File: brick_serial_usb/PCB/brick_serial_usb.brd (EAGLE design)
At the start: 27.9 x 39.4 mm, 15 parts, among them U1 FT232RL-SSOP28

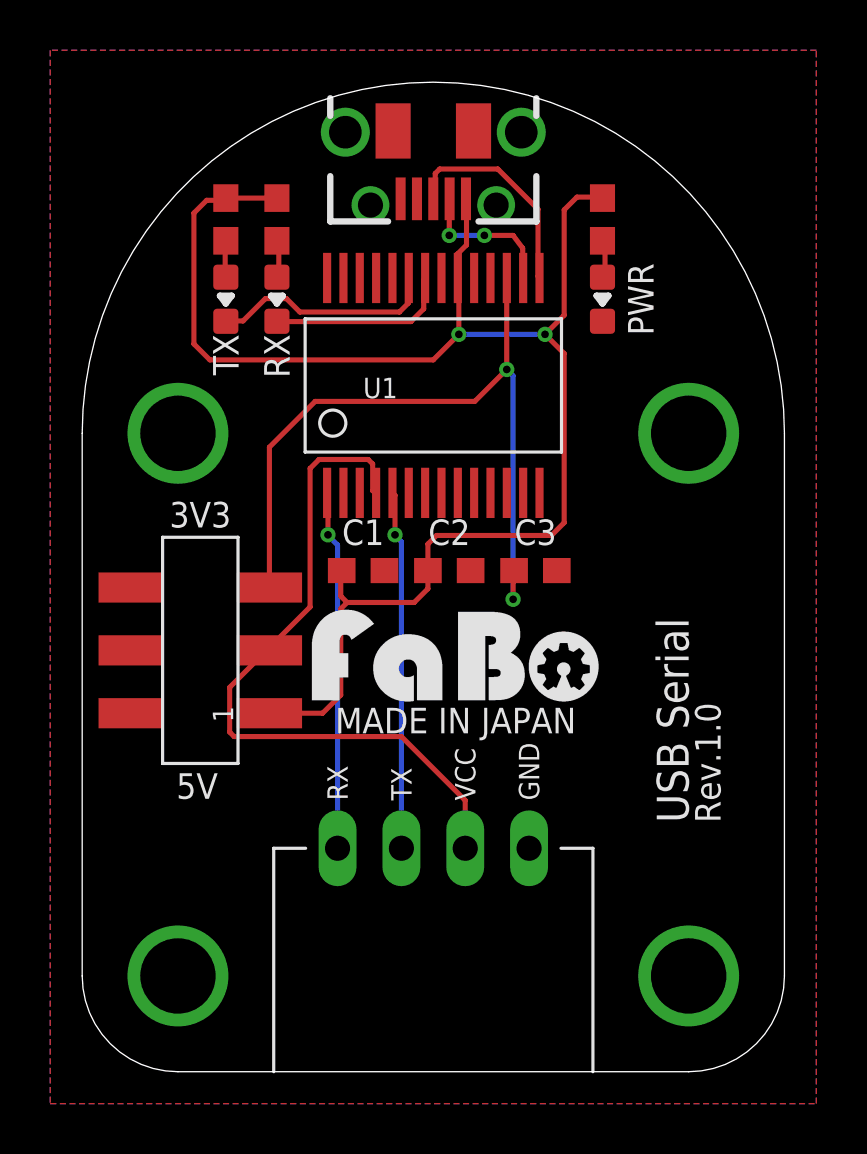
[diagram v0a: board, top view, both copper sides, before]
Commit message: refine board brick_serial_usb
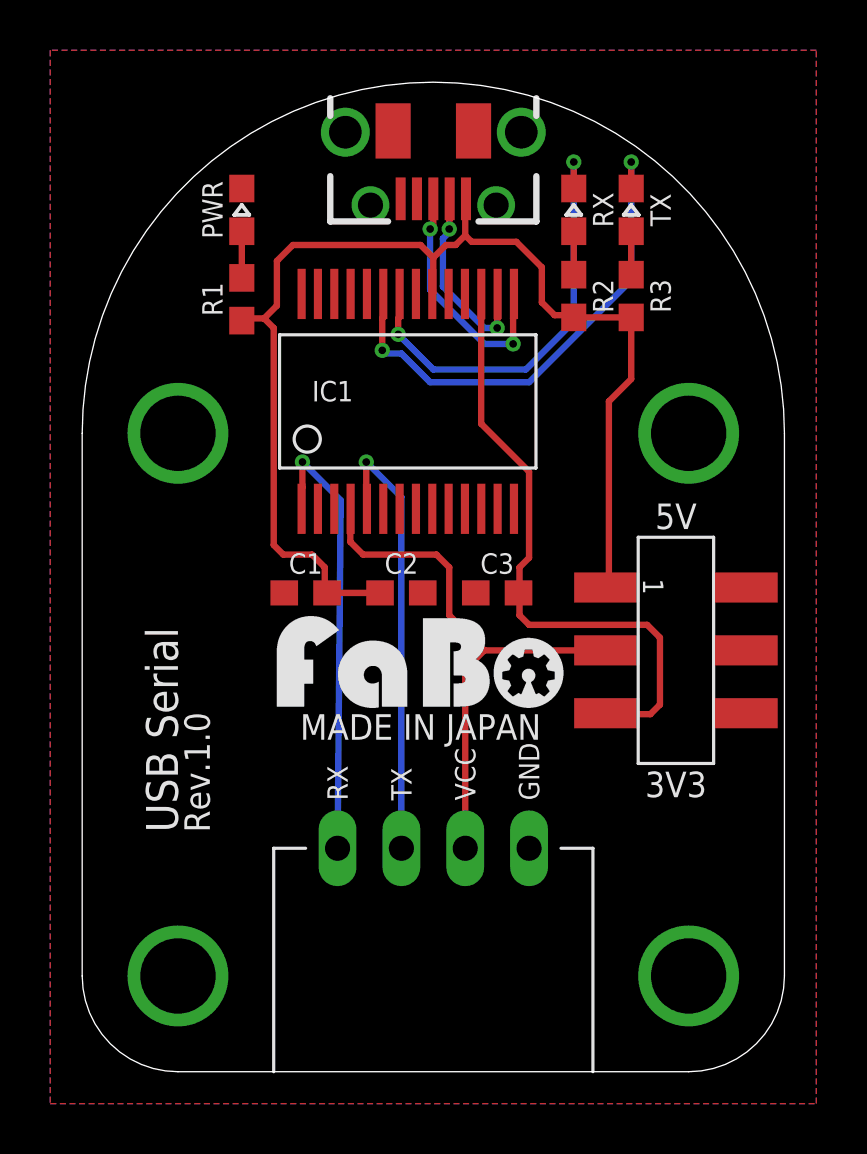
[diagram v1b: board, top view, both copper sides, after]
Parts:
- removed U1: FT232RL-SSOP28, gclue:SSOP28
- added IC1: FT232RL-SSOP28, FaBo-etc:SSOP28
- C1, C2, C3: device gclue:EIA0603 -> FaBo-etc:EIA0603
- J1: device FaBo-etc:BRICK_SERIAL -> FaBo-Template:FABO_BRICK_SERIAL
- JP1: device gclue:USB_B_MICRO -> FaBo-etc:USB_B_MICRO
- PWR, RX, TX: device gclue:EIA0603-LED -> FaBo-etc:EIA0603-LED
- R1, R2, R3: value (none) -> 220; device gclue:EIA0603 -> FaBo-etc:EIA0603
- SW1: device gclue:C&K_JS202011SCQN -> FaBo-etc:C&K_JS202011SCQN
- U$5: device FaBo:LOGO_FABO_M -> FaBo-etc:LOGO_OSHW_T_M_BOTTOM
- U$6: device gclue:LOGO_OSHW_T_M_BOTTOM -> FaBo-etc:LOGO_FABO_M
- moved SW1 18.9 mm to (23.6, 16.8), turned to 0 degrees
- moved TX 16.5 mm to (21.8, 34.3), turned to 90 degrees
- moved PWR 14.8 mm to (6.35, 34.3), turned to 90 degrees
- moved R1 14.7 mm to (6.35, 30.7), turned to 270 degrees
- moved R3 14.4 mm to (21.8, 30.9), turned to 270 degrees
- moved R2 14.2 mm to (19.6, 30.9), turned to 270 degrees
- moved RX 12.3 mm to (19.6, 34.3), turned to 90 degrees
- moved U$5 9.95 mm to (14.0, 4.83)
- moved U$6 9.16 mm to (13.5, 14.5)
- moved C1 2.45 mm to (8.89, 19.1), turned to 180 degrees
- moved C2 2.10 mm to (12.7, 19.1)
- moved C3 1.76 mm to (16.5, 19.1), turned to 180 degrees
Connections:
- removed net N$4: JP1.D-, U1.16
- removed net N$5: JP1.D+, U1.15
- new net USBDM: IC1.16, JP1.D-
- new net USBDP: IC1.15, JP1.D+
- net 3V3: now also IC1.17; no longer U1.17
- net 5V: now also IC1.20; no longer U1.20
- net GND: now also IC1.18, IC1.21, IC1.25, IC1.26, IC1.7; no longer U1.18, U1.21, U1.25, U1.26, U1.7
- net N$2: now also R3.1; no longer R2.1
- net N$3: now also R2.1; no longer R3.1
- net RX: now also IC1.1; no longer U1.1
- net RXLED: now also IC1.22; no longer U1.22
- net TX: now also IC1.5; no longer U1.5
- net TXLED: now also IC1.23; no longer U1.23
- net VCC: now also IC1.4; no longer U1.4
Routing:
- net 5V: track 63.1 -> 49.3 mm, vias 2 -> 0
- net TXLED: track 9.00 -> 20.1 mm, vias 0 -> 2
- net RXLED: track 7.30 -> 17.4 mm, vias 0 -> 2
- net USBDP: track 0.00 -> 9.86 mm, vias 0 -> 2
- net N$5: track 8.61 -> 0.00 mm
- net USBDM: track 0.00 -> 7.80 mm, vias 0 -> 2
- net N$4: track 5.82 -> 0.00 mm, vias 2 -> 0
- net 3V3: track 30.4 -> 24.7 mm, vias 2 -> 0
- net VCC: track 28.2 -> 22.6 mm
- net RX: track 14.3 -> 17.9 mm
- net TX: track 14.3 -> 17.8 mm
